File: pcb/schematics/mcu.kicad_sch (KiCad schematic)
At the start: 25 parts, among them J3 Conn_01x06_Female, SW2 Reset, U3 STM32F103V8Tx, Y2 24MHz

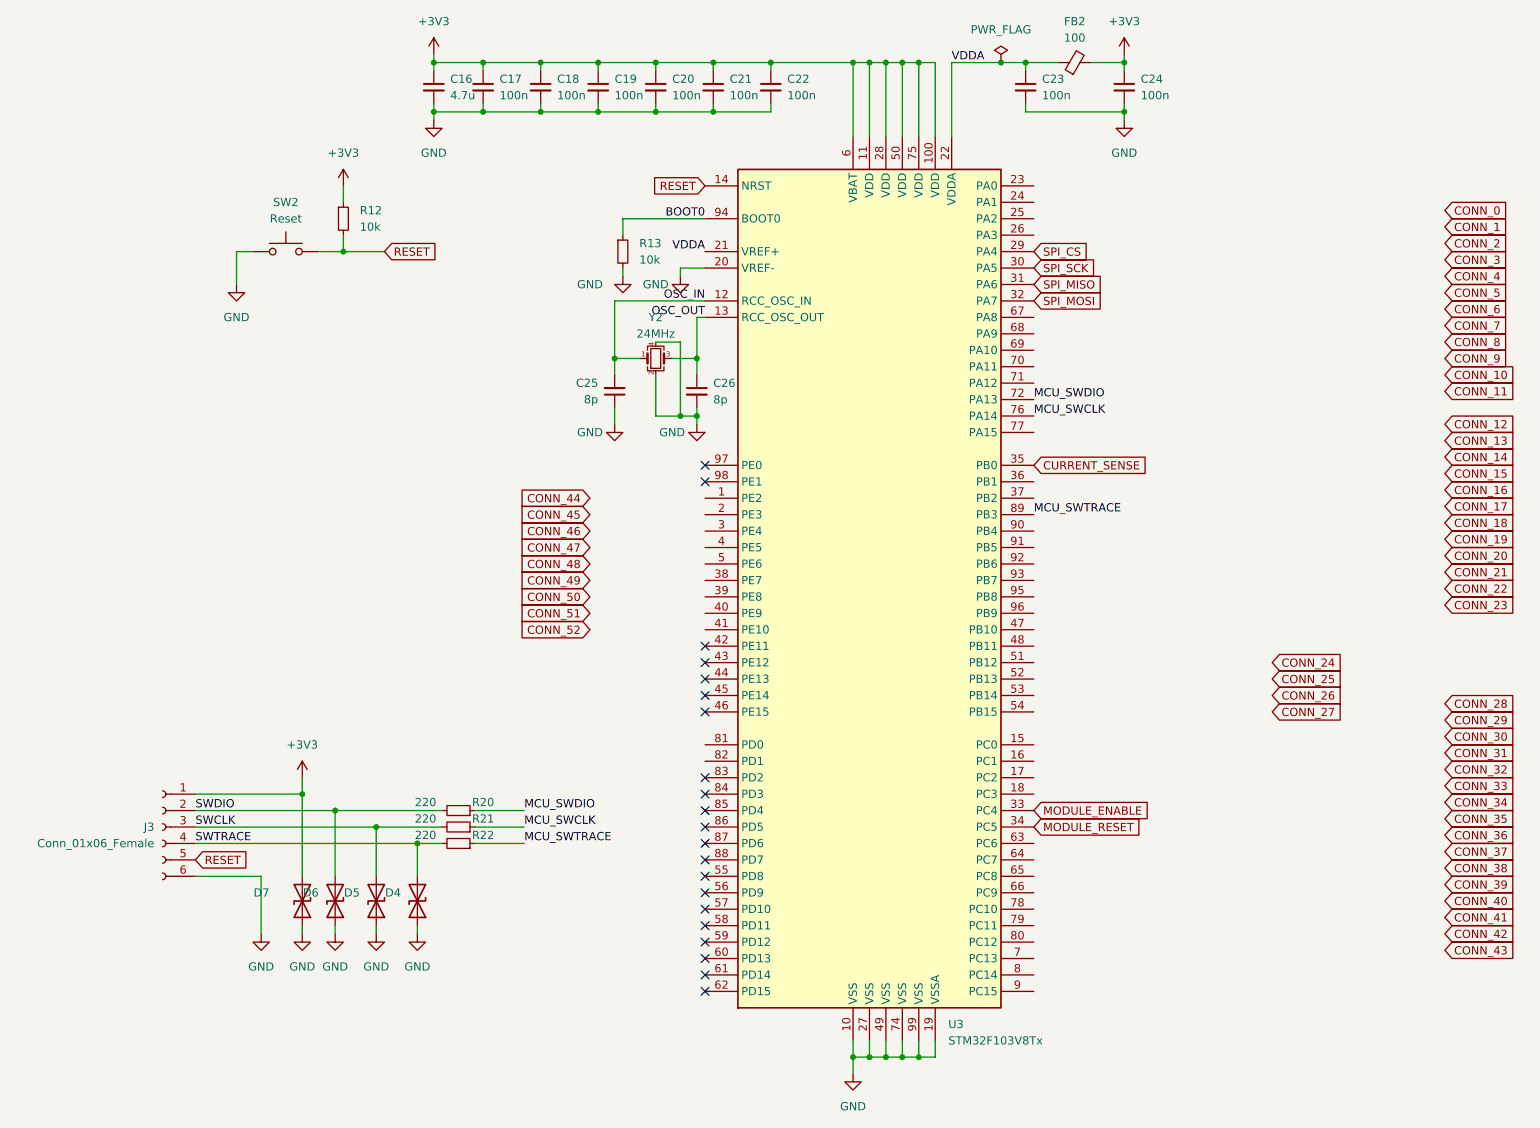
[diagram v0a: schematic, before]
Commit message: add bus traces
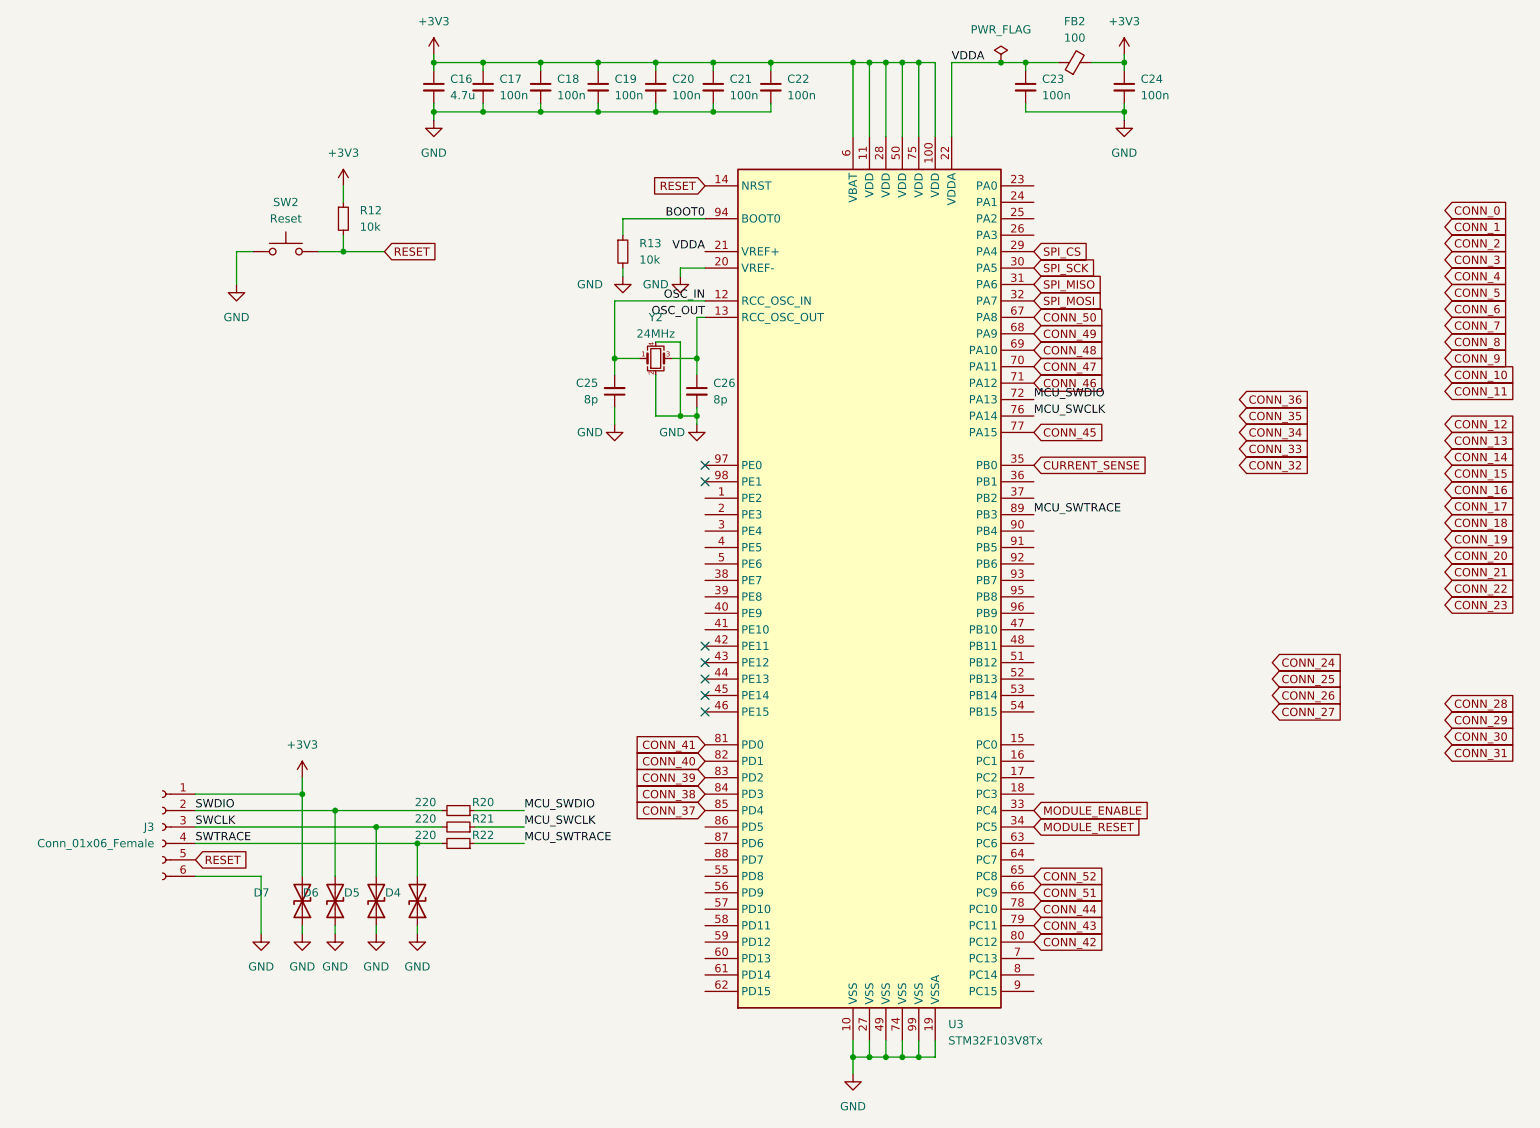
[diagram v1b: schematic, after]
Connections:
- net CONN_37: now also U3.85 (PD4)
- net CONN_38: now also U3.84 (PD3)
- net CONN_39: now also U3.83 (PD2)
- net CONN_40: now also U3.82 (PD1)
- net CONN_41: now also U3.81 (PD0)
- net CONN_42: now also U3.80 (PC12)
- net CONN_43: now also U3.79 (PC11)
- net CONN_44: now also U3.78 (PC10)
- net CONN_45: now also U3.77 (PA15)
- net CONN_46: now also U3.71 (PA12)
- net CONN_47: now also U3.70 (PA11)
- net CONN_48: now also U3.69 (PA10)
- net CONN_49: now also U3.68 (PA9)
- net CONN_50: now also U3.67 (PA8)
- net CONN_51: now also U3.66 (PC9)
- net CONN_52: now also U3.65 (PC8)
- no-connect marks 21 -> 7
